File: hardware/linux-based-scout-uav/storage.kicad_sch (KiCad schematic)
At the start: 8 parts, among them J2 Micro_SD_Card_Det2, U8 EMMC04G-W627-M06U

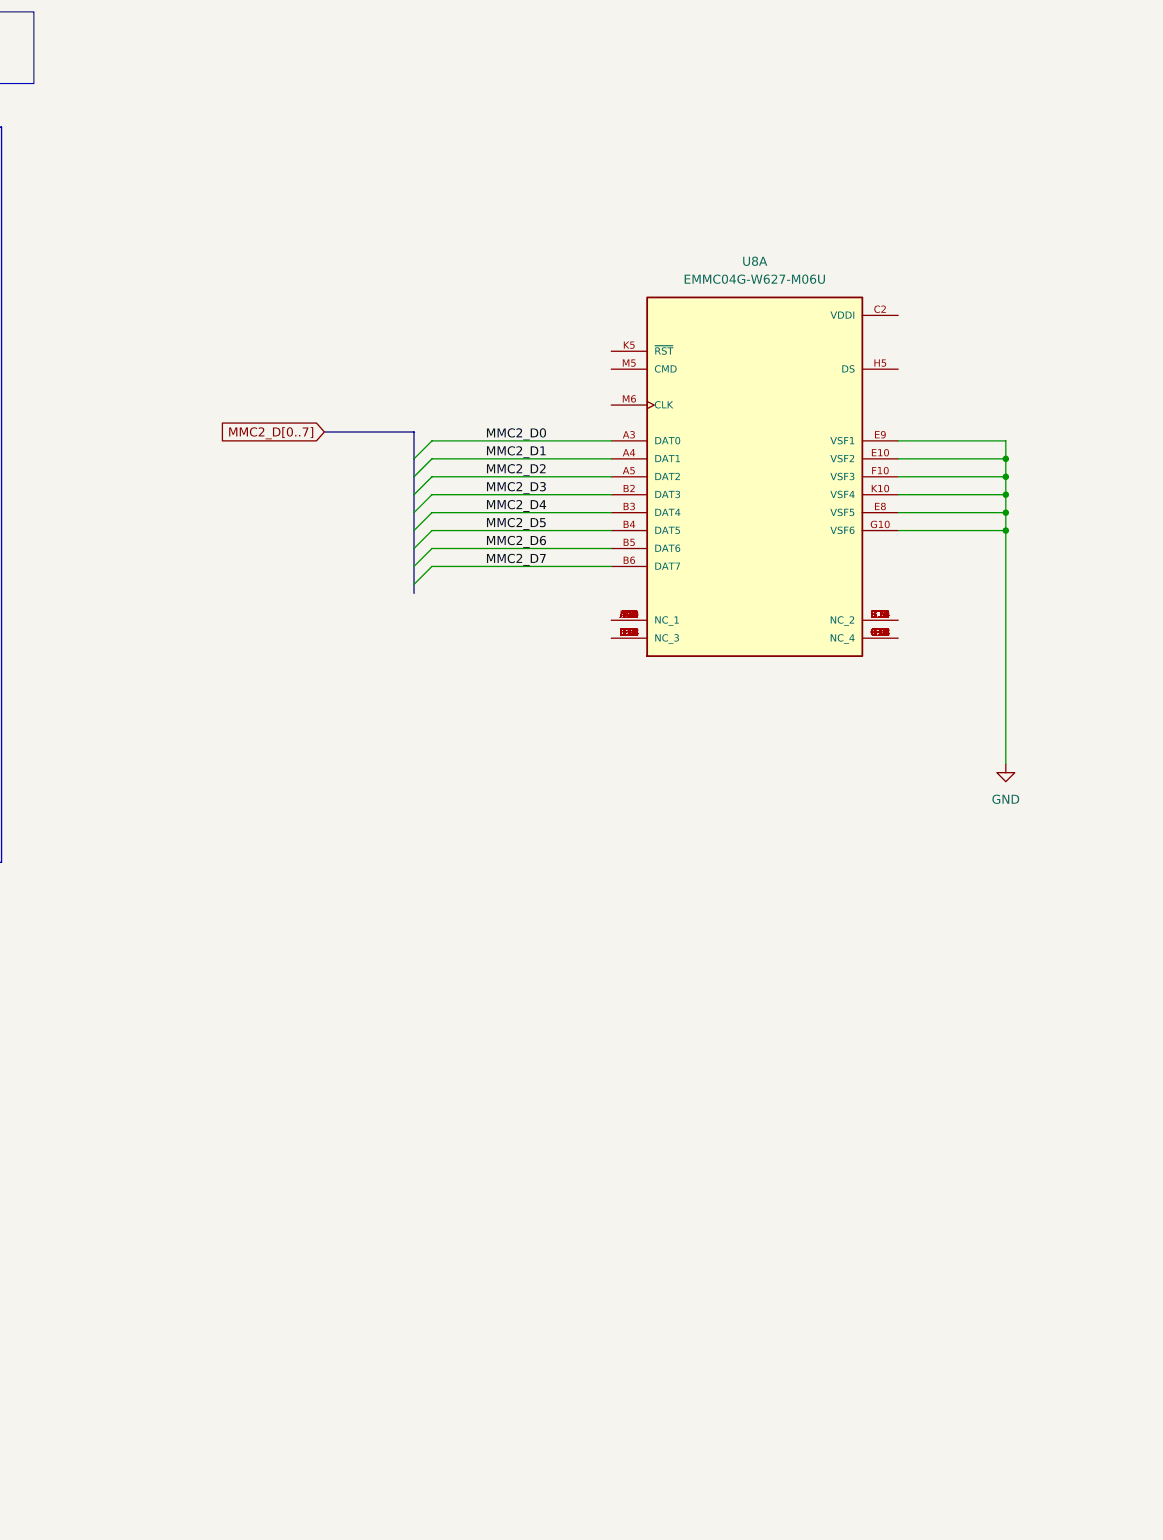
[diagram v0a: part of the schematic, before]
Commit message: Schematic update
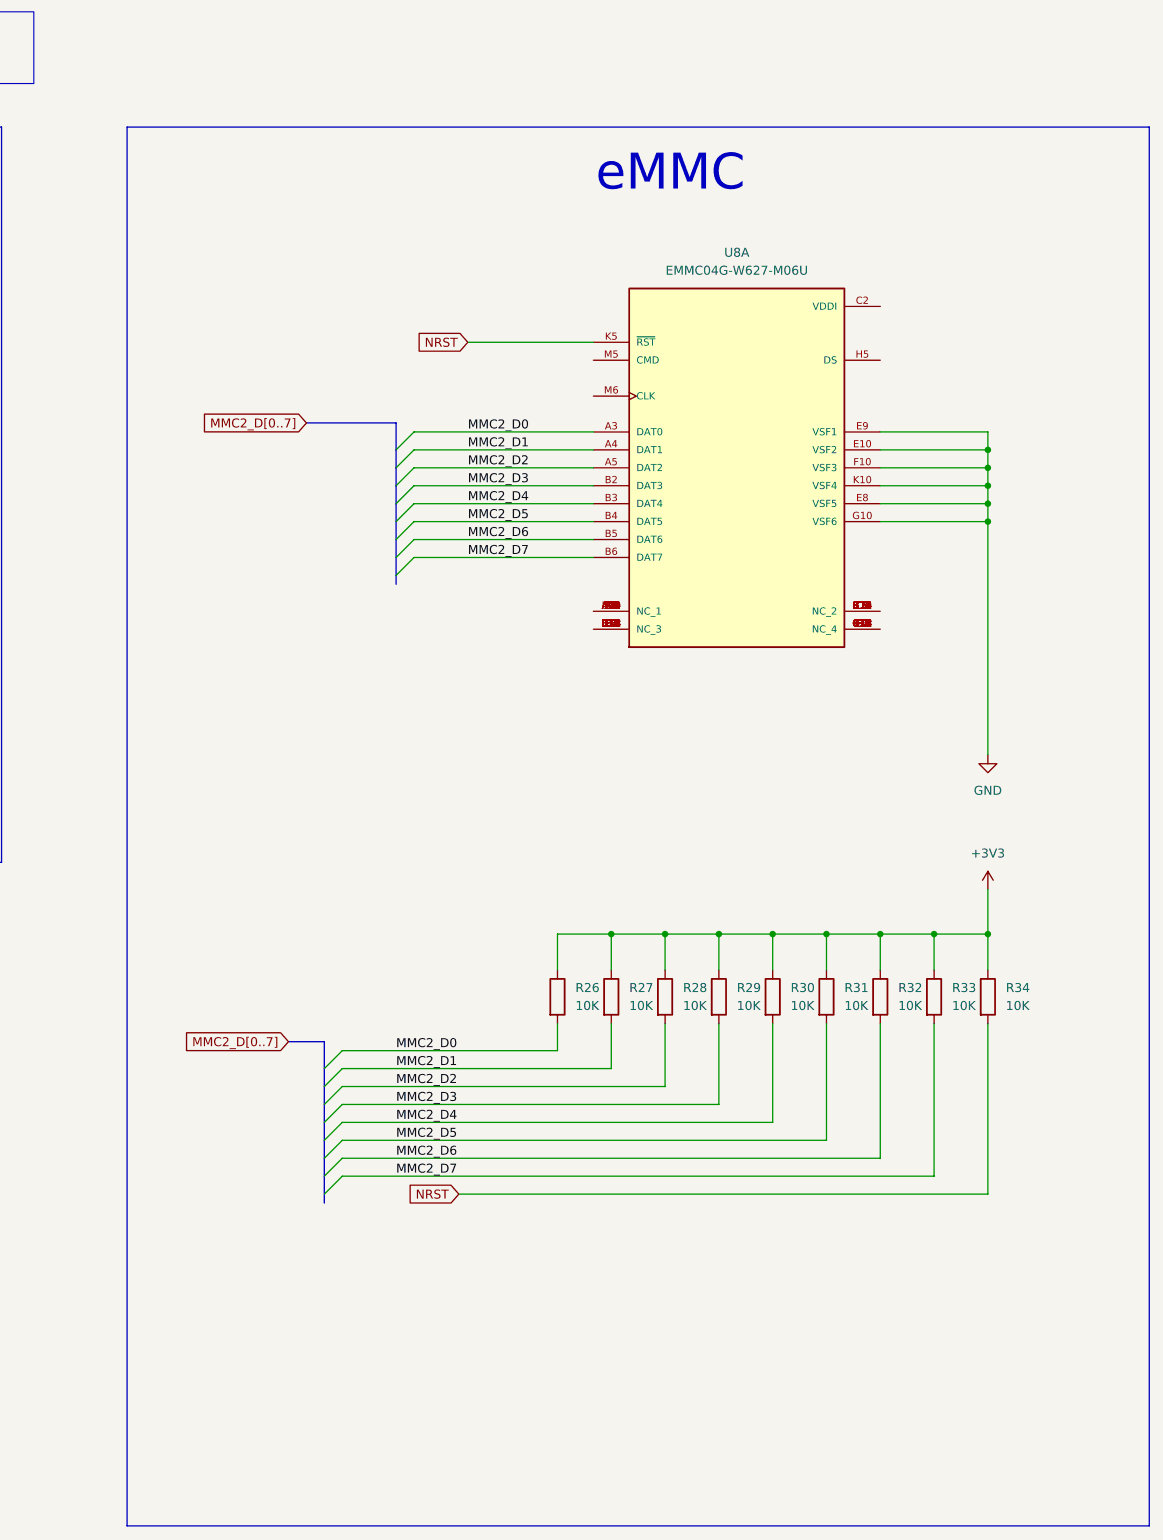
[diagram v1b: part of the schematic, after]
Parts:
- added R26, R27, R28, R29, R30, R31, R32, R33, R34: 10K, symbol Device:R
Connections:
- net +3V3: now also R26.1, R27.1, R28.1, R29.1, R30.1, R31.1, R32.1, R33.1, R34.1
- net MMC2_D0: now also R26.2
- net MMC2_D1: now also R27.2
- net MMC2_D2: now also R28.2
- net MMC2_D3: now also R29.2
- net MMC2_D4: now also R30.2
- net MMC2_D5: now also R31.2
- net MMC2_D6: now also R32.2
- net MMC2_D7: now also R33.2
- net NRST: now reaches U8.K5 (~{RST})
- net NRST: now also R34.2
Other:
- note added: "eMMC"
- moved on the sheet: U8A
